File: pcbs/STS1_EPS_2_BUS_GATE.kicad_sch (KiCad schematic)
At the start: 20 parts, among them Q5 SI7135DP-T1-GE3, Q6 SI7135DP-T1-GE3, Q7 SI7135DP-T1-GE3, Q8 SI7135DP-T1-GE3, Q9 SI7135DP-T1-GE3, U3 TPS2420RSAT

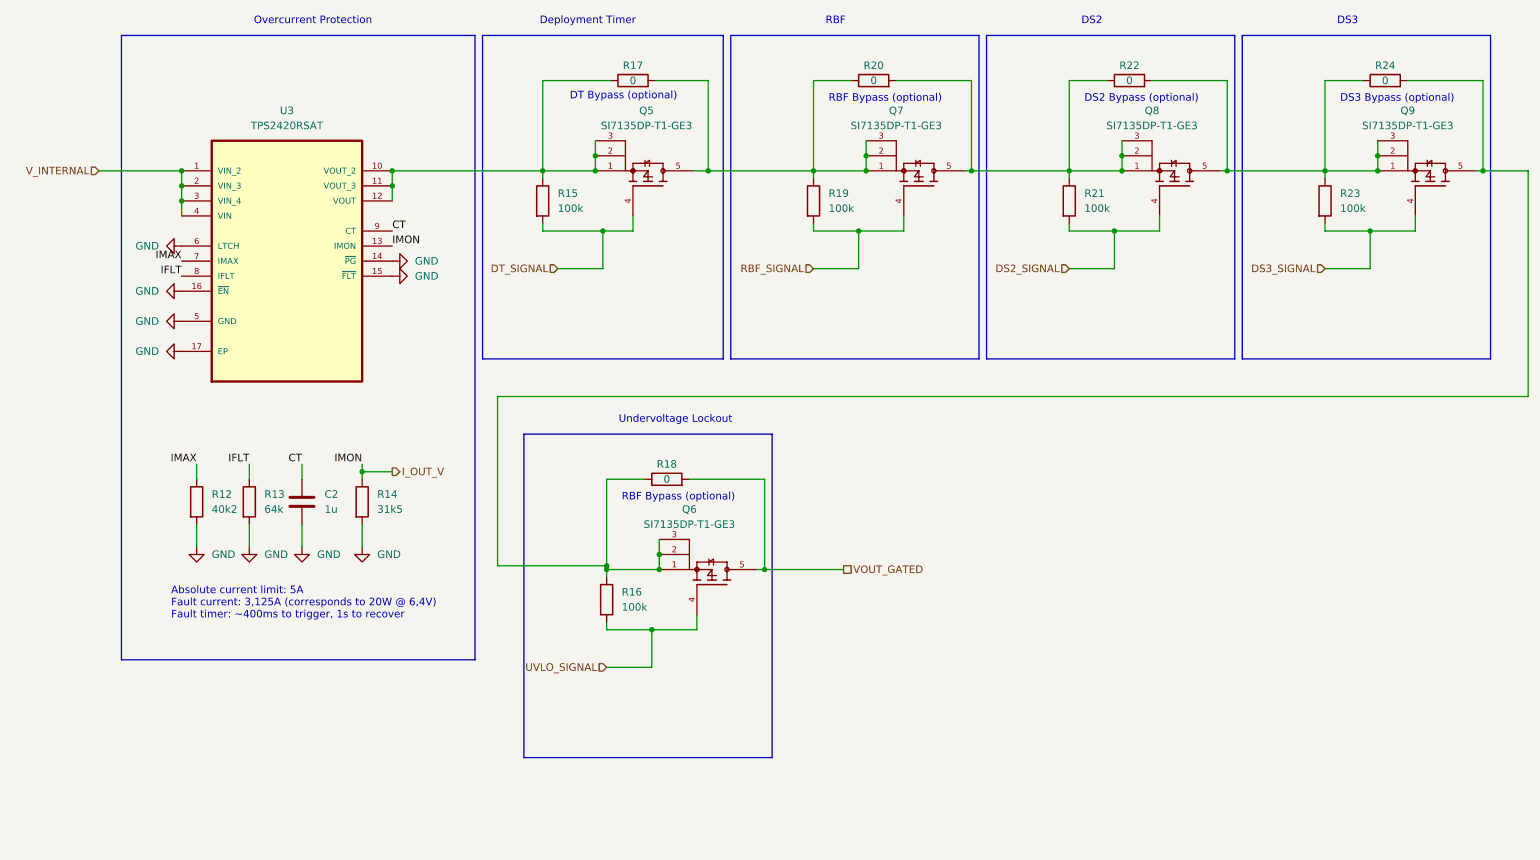
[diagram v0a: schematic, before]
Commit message: Worked on STS1_EPS_2.
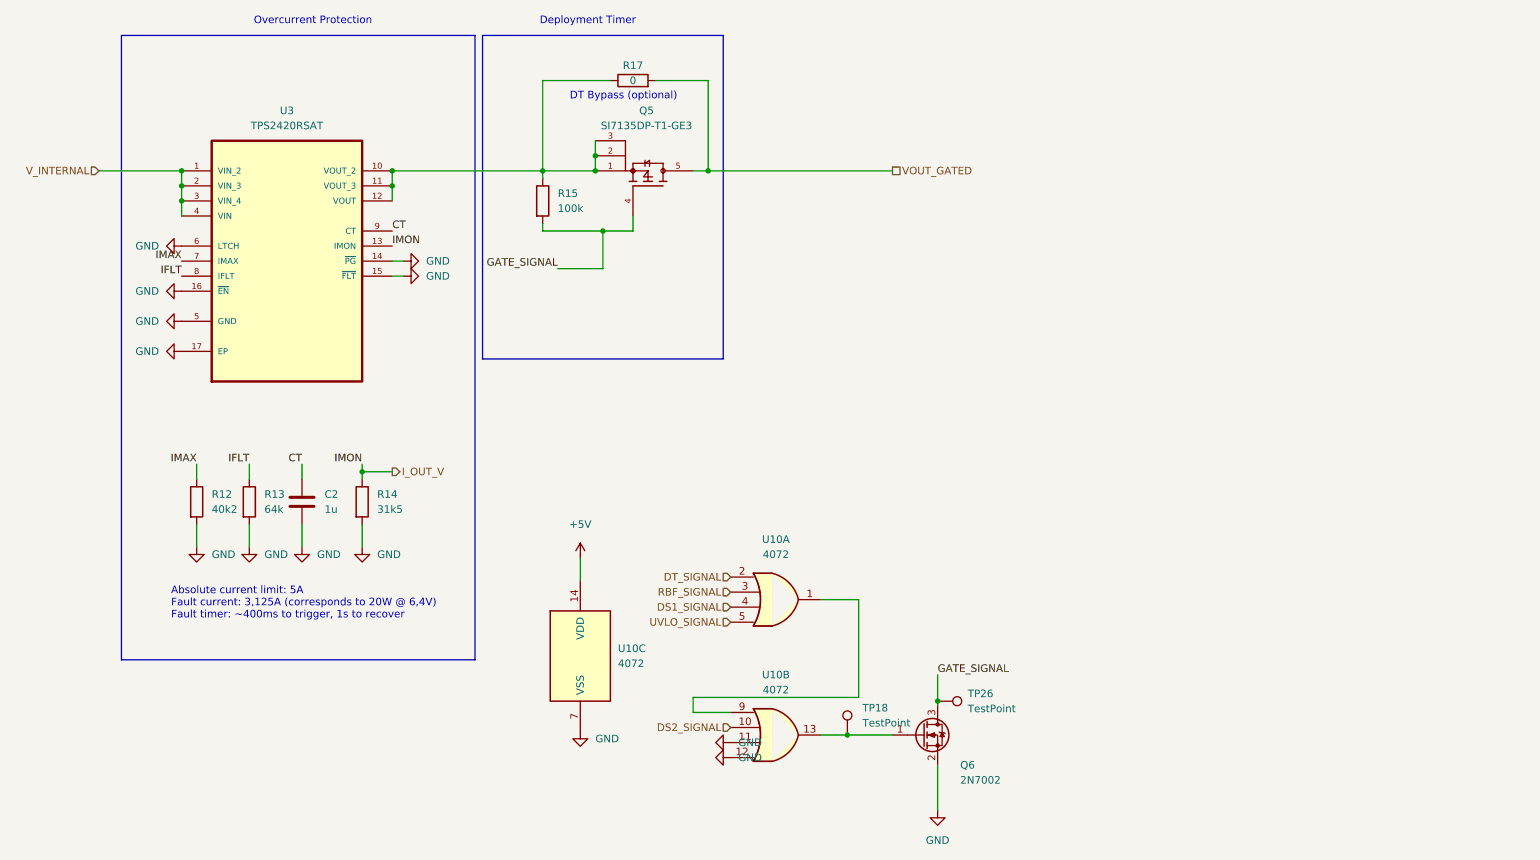
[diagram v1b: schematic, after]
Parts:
- removed Q6, Q7, Q8, Q9: SI7135DP-T1-GE3, STS_Package_SO:POWERPAK_SO8_single, symbol STS_Transistor_FET:SI7135DP-T1-GE3
- removed R16, R19, R21, R23: 100k, Resistor_SMD:R_0805_2012Metric, symbol Device:R
- removed R18, R20, R22, R24: 0, Resistor_SMD:R_0805_2012Metric, symbol Device:R
- added Q6: 2N7002, Package_TO_SOT_SMD:SOT-23, symbol Transistor_FET:2N7002
- added TP18, TP26: TestPoint, TestPoint:TestPoint_THTPad_D1.0mm_Drill0.5mm, symbol Connector:TestPoint
- added U10: 4072, Package_SO:SOIC-14_3.9x8.7mm_P1.27mm, symbol 4xxx:4072
- U3: footprint Package_DFN_QFN:VQFN-16-1EP_3x3mm_P0.5mm_EP1.45x1.45mm_ThermalVias -> STS_Package_DFN_QFN:QFN65P400X400X100-17N
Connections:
- net DS2_SIGNAL: now also U10.10
- net DT_SIGNAL: now also U10.2; no longer Q5.4, R15.2
- net GND: now also Q6.2 (S), U10.11, U10.12, U10.7 (VSS)
- net RBF_SIGNAL: now also U10.3
- net UVLO_SIGNAL: now also U10.5
- net VOUT_GATED: now also Q5.5, R17.2
- new net: Q6.1 (G), TP18.1, U10.13
- new net: U10.1, U10.9
- new net +5V: U10.14 (VDD)
- new net DS1_SIGNAL: U10.4
- new net GATE_SIGNAL: Q5.4, Q6.3 (D), R15.2, TP26.1
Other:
- note removed: "DS2"
- note removed: "DS2 Bypass (optional)"
- note removed: "DS3"
- note removed: "DS3 Bypass (optional)"
- note removed: "RBF"
- note removed: "RBF Bypass (optional)"
- note removed: "Undervoltage Lockout"
